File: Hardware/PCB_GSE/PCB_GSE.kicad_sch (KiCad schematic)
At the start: 37 parts, among them J1 Conn_01x06_Pin, U1 STM32F103CBT6

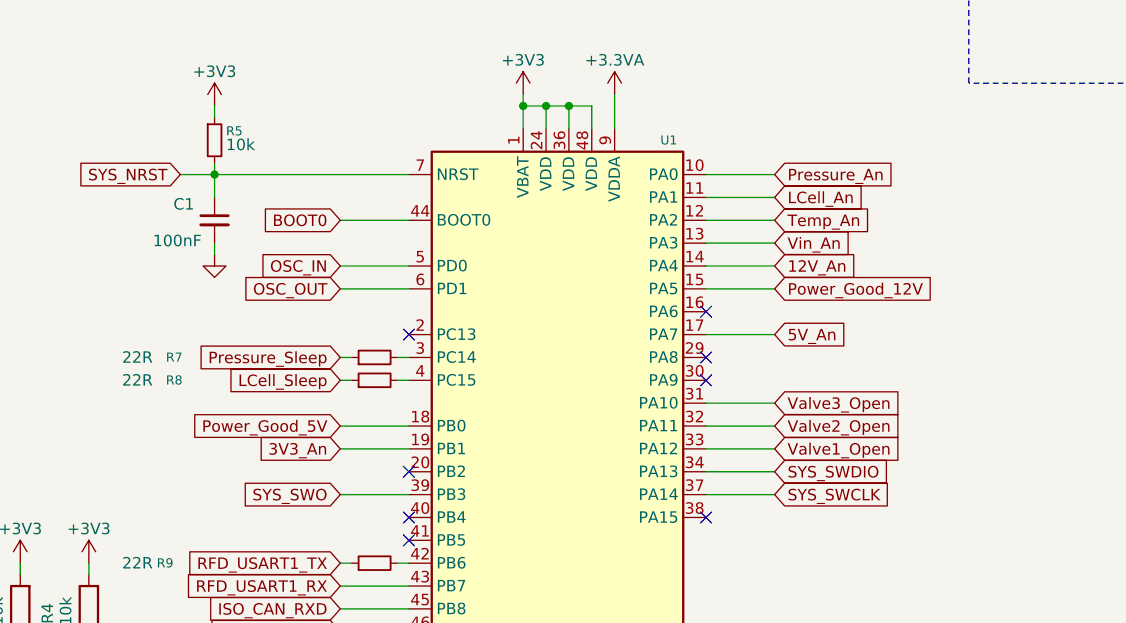
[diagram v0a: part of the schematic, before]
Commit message: wip : Done routing
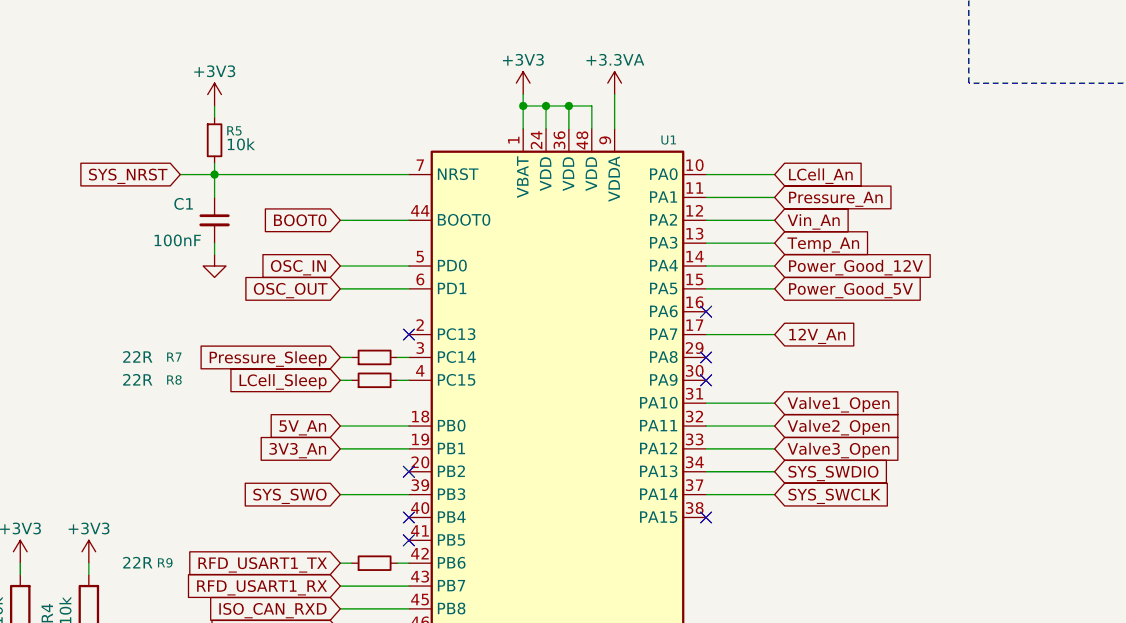
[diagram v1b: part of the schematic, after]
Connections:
- net 12V_An: now also U1.17 (PA7); no longer U1.14 (PA4)
- net 5V_An: now also U1.18 (PB0); no longer U1.17 (PA7)
- net LCell_An: now also U1.10 (PA0); no longer U1.11 (PA1)
- net Power_Good_12V: now also U1.14 (PA4); no longer U1.15 (PA5)
- net Power_Good_5V: now also U1.15 (PA5); no longer U1.18 (PB0)
- net Pressure_An: now also U1.11 (PA1); no longer U1.10 (PA0)
- net Temp_An: now also U1.13 (PA3); no longer U1.12 (PA2)
- net Valve1_Open: now also U1.31 (PA10); no longer U1.33 (PA12)
- net Valve3_Open: now also U1.33 (PA12); no longer U1.31 (PA10)
- net Vin_An: now also U1.12 (PA2); no longer U1.13 (PA3)
